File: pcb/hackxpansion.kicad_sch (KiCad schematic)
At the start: 0 parts

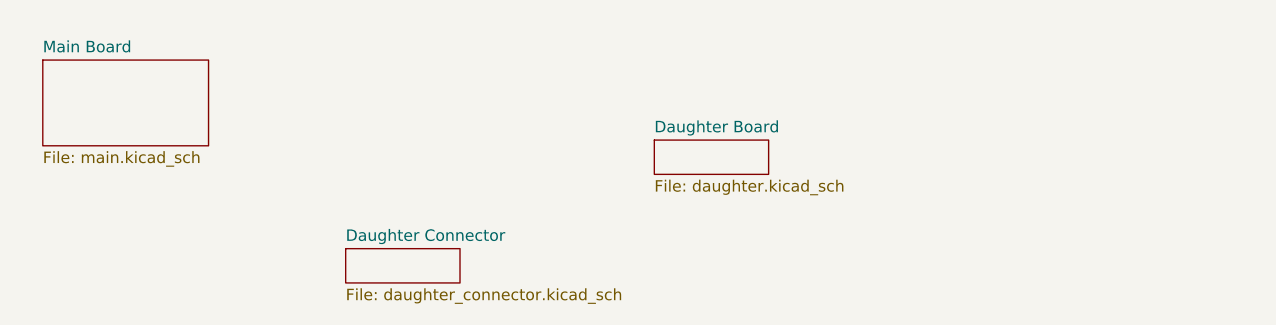
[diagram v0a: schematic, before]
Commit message: moved stuff around
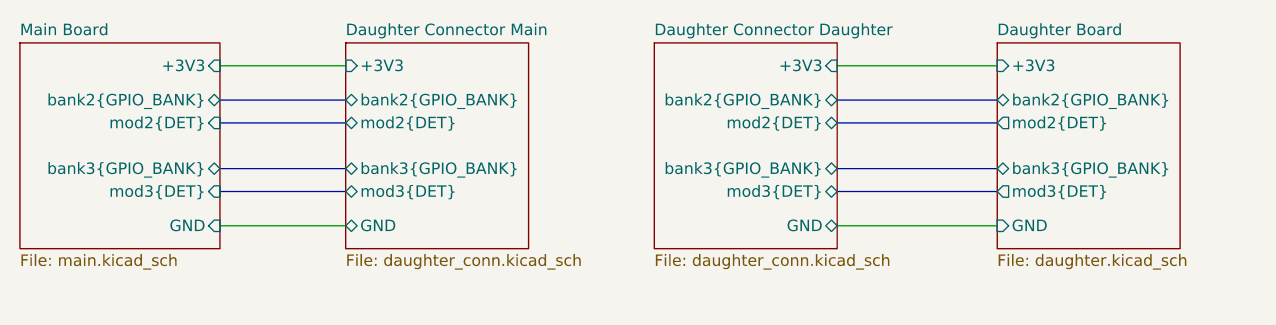
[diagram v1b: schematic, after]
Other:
- sheet Daughter Connector renamed Daughter Connector Main
- added sheet Daughter Connector Daughter (daughter_conn.kicad_sch)
- sheet Daughter Board ports: added +3V3, GND, bank2{GPIO_BANK}, bank3{GPIO_BANK}, mod2{DET}, mod3{DET}; removed none
- sheet Daughter Connector Main: file daughter_connector.kicad_sch -> daughter_conn.kicad_sch
- sheet Daughter Connector Main ports: added +3V3, GND, bank2{GPIO_BANK}, bank3{GPIO_BANK}, mod2{DET}, mod3{DET}; removed none
- sheet Main Board ports: added +3V3, GND, bank2{GPIO_BANK}, bank3{GPIO_BANK}, mod2{DET}, mod3{DET}; removed none
